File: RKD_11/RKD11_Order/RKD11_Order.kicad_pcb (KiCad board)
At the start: 2 copper layers, 99.4 x 99.4 mm, 140 parts, among them J1 Conn_01x06, J3 Qwiic_RA, SW1 RotaryEncoder_Switch, SW2 SW_Push, SW99 KEY_SWITCH, U1 ProMicro

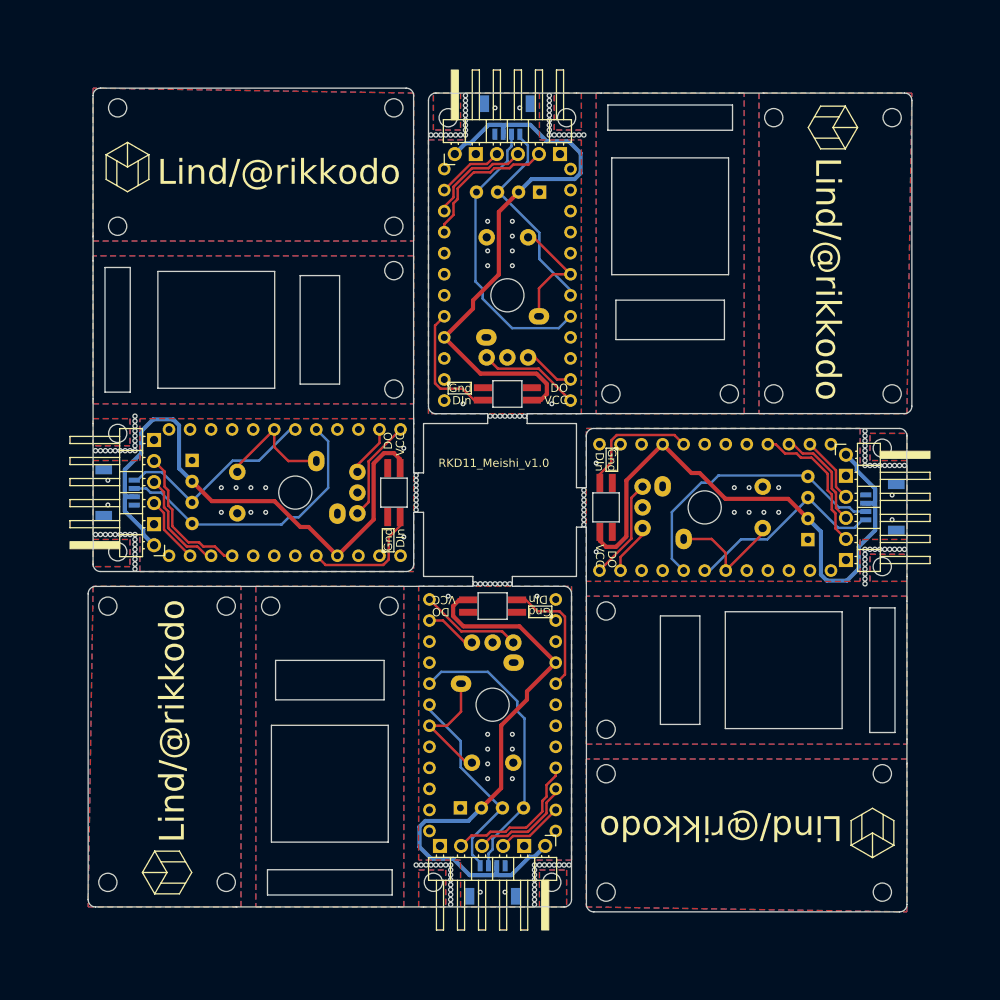
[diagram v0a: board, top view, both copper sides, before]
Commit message: Update
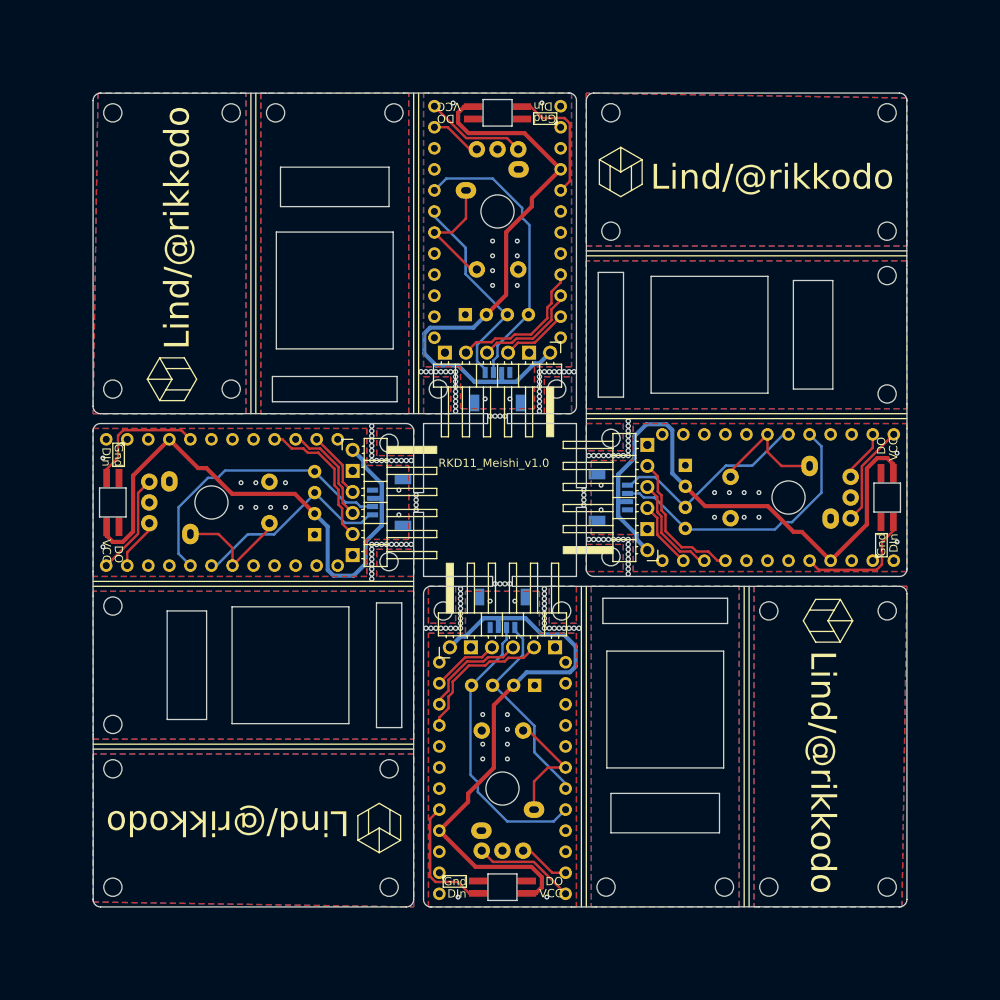
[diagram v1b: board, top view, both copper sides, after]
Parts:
- removed the J1 at (131.8, 58.0)
- removed the J1 at (95.5, 105.2)
- removed the J1 at (142.7, 141.5)
- removed the J1 at (179.0, 94.3)
- removed the J3 at (93.1, 98.8)
- removed the J3 at (181.4, 100.6)
- removed the J3 at (138.1, 55.6)
- removed the J3 at (136.3, 143.9)
- removed the LED1 at (124.4, 98.8)
- removed the LED1 at (138.1, 86.9)
- removed the LED1 at (136.3, 112.5)
- removed the LED1 at (150.0, 100.6)
- removed the LED3 at (157.8, 53.6)
- removed the LED3 at (91.1, 79.2)
- removed the LED3 at (116.7, 145.9)
- removed the LED3 at (183.4, 120.3)
- removed the OL1 at (192.9, 100.7)
- removed the OL1 at (138.2, 44.1)
- removed the OL1 at (136.2, 155.4)
- removed the OL1 at (81.6, 98.7)
- removed the REF** at (184.5, 105.7)
- removed the REF** at (143.2, 54.8)
- removed the REF** at (127.4, 143.8)
- removed the REF** at (93.2, 106.6)
- removed the REF** at (132.8, 55.7)
- removed the REF** at (127.1, 98.8)
- removed the REF** at (182.2, 105.7)
- removed the REF** at (92.3, 93.8)
- removed the REF** at (133.1, 53.6)
- removed the REF** at (181.3, 108.3)
- removed the REF** at (133.1, 52.4)
- removed the REF** at (185.7, 105.7)
- removed the REF** at (133.1, 51.2)
- removed the REF** at (93.2, 93.5)
- removed the REF** at (92.3, 59.5)
- removed the REF** at (145.3, 143.8)
- removed the REF** at (130.4, 55.7)
- removed the REF** at (182.2, 95.5)
- removed the REF** at (131.0, 143.8)
- removed the REF** at (144.7, 55.7)
- removed the REF** at (142.9, 143.8)
- removed the REF** at (131.3, 145.9)
- removed the REF** at (185.7, 95.5)
- removed the REF** at (89.9, 93.8)
- removed the REF** at (91.1, 93.8)
- removed the REF** at (93.2, 92.3)
- removed the REF** at (97.0, 144.7)
- removed the REF** at (181.3, 106.0)
- removed the REF** at (131.3, 144.7)
- removed the REF** at (136.3, 109.8)
- removed the REF** at (133.1, 54.8)
- removed the REF** at (181.3, 91.7)
- removed the REF** at (181.3, 107.2)
- removed the REF** at (143.2, 52.4)
- removed the REF** at (141.7, 143.8)
- removed the REF** at (131.3, 148.2)
- removed the REF** at (138.1, 89.6)
- removed the REF** at (141.4, 148.2)
- removed the REF** at (143.2, 51.2)
- removed the REF** at (89.9, 103.9)
- removed the REF** at (147.3, 100.6)
- removed the REF** at (131.3, 147.0)
- removed the REF** at (92.3, 103.9)
- removed the REF** at (141.4, 145.9)
- removed the REF** at (177.4, 54.8)
- removed the REF** at (183.4, 105.7)
- removed the REF** at (145.9, 55.7)
- removed the REF** at (181.3, 109.5)
- removed the REF** at (131.6, 55.7)
- removed the REF** at (181.3, 92.9)
- removed the REF** at (183.4, 95.5)
- removed the REF** at (144.1, 143.8)
- removed the REF** at (88.7, 103.9)
- removed the REF** at (181.3, 94.1)
- removed the REF** at (141.4, 147.0)
- removed the REF** at (141.4, 144.7)
- removed the REF** at (93.2, 91.1)
- removed the REF** at (93.2, 104.2)
- removed the REF** at (129.8, 143.8)
- removed the REF** at (181.3, 95.2)
- removed the REF** at (143.2, 53.6)
- removed the REF** at (129.2, 55.7)
- removed the REF** at (143.5, 55.7)
- removed the REF** at (182.2, 139.9)
- removed the REF** at (128.6, 143.8)
- removed the REF** at (91.1, 103.9)
- removed the REF** at (147.0, 55.7)
- removed the REF** at (88.7, 93.8)
- removed the REF** at (93.2, 89.9)
- removed the REF** at (184.5, 95.5)
- removed the REF** at (93.2, 107.8)
- removed the REF** at (93.2, 105.4)
- removed the Ref** at (184.5, 86.9)
- removed the Ref** at (170.3, 53.6)
- removed the Ref** at (150.6, 86.9)
- removed the Ref** at (124.4, 66.7)
- removed the Ref** at (91.1, 106.0)
- removed the Ref** at (184.5, 53.6)
- removed the Ref** at (150.0, 147.0)
- removed the Ref** at (183.4, 147.0)
- removed the Ref** at (170.3, 86.9)
- removed the Ref** at (91.1, 66.7)
- removed the Ref** at (89.9, 145.9)
- removed the Ref** at (150.0, 132.8)
- removed the Ref** at (124.4, 86.3)
- removed the Ref** at (143.5, 145.9)
- removed the Ref** at (123.8, 112.5)
- removed the Ref** at (124.4, 52.4)
- removed the Ref** at (131.0, 53.6)
- removed the Ref** at (150.0, 127.4)
- removed the Ref** at (145.3, 53.6)
- removed the Ref** at (164.9, 86.9)
- removed the Ref** at (91.1, 91.7)
- removed the Ref** at (109.5, 112.5)
- removed the Ref** at (104.2, 112.5)
- removed the Ref** at (150.0, 113.1)
- removed the Ref** at (183.4, 107.8)
- removed the Ref** at (129.2, 145.9)
- removed the Ref** at (124.4, 72.0)
- removed the Ref** at (89.9, 112.5)
- removed the Ref** at (104.2, 145.9)
- removed the Ref** at (183.4, 93.5)
- removed the Ref** at (91.1, 52.4)
- removed the Ref** at (183.4, 132.8)
- removed the SW1 at (138.1, 75.0)
- removed the SW1 at (112.5, 98.8)
- removed the SW1 at (161.9, 100.6)
- removed the SW1 at (136.3, 124.4)
- removed the SW2 at (161.9, 100.6)
- removed the SW2 at (112.5, 98.8)
- removed the SW2 at (136.3, 124.4)
- removed the SW2 at (138.1, 75.0)
- removed the SW99 at (103.0, 79.2)
- removed the SW99 at (116.7, 134.0)
- removed the SW99 at (171.5, 120.3)
- removed the SW99 at (157.8, 65.5)
- removed the U1 at (136.3, 124.4)
- removed the U1 at (112.5, 98.8)
- removed the U1 at (161.9, 100.6)
- removed the U1 at (138.1, 75.0)
- added J1: Conn_01x06, Connector_PinHeader_2.54mm:PinHeader_1x06_P2.54mm_Horizontal, F.Cu at (155.0, 105.8)
- added J1: Conn_01x06, Connector_PinHeader_2.54mm:PinHeader_1x06_P2.54mm_Horizontal, F.Cu at (119.4, 93.7)
- added J1: Conn_01x06, Connector_PinHeader_2.54mm:PinHeader_1x06_P2.54mm_Horizontal, F.Cu at (131.2, 117.5)
- added J1: Conn_01x06, Connector_PinHeader_2.54mm:PinHeader_1x06_P2.54mm_Horizontal, F.Cu at (143.3, 81.9)
- added J3: Qwiic_RA, SparkFun-Connector:JST_SMD_1.0mm-4_Black, B.Cu at (137.5, 115.1)
- added J3: Qwiic_RA, SparkFun-Connector:JST_SMD_1.0mm-4_Black, B.Cu at (121.8, 100.0)
- added J3: Qwiic_RA, SparkFun-Connector:JST_SMD_1.0mm-4_Black, B.Cu at (136.9, 84.3)
- added J3: Qwiic_RA, SparkFun-Connector:JST_SMD_1.0mm-4_Black, B.Cu at (152.6, 99.4)
- added LED1: LED_SK6812MINI-E, kbd_Parts:LED_SK6812MINI-E_UG, B.Cu at (136.9, 53.0)
- added LED1: LED_SK6812MINI-E, kbd_Parts:LED_SK6812MINI-E_UG, B.Cu at (90.5, 100.0)
- added LED1: LED_SK6812MINI-E, kbd_Parts:LED_SK6812MINI-E_UG, B.Cu at (137.5, 146.4)
- added LED1: LED_SK6812MINI-E, kbd_Parts:LED_SK6812MINI-E_UG, B.Cu at (184.0, 99.4)
- added LED3: LED_SK6812MINI-E, Rikkodo_FootPrint:rkd_KeyHall_3ox15, F.Cu at (123.8, 119.7)
- added LED3: LED_SK6812MINI-E, Rikkodo_FootPrint:rkd_KeyHall_3ox15, F.Cu at (117.3, 86.3)
- added LED3: LED_SK6812MINI-E, Rikkodo_FootPrint:rkd_KeyHall_3ox15, F.Cu at (150.6, 79.8)
- added LED3: LED_SK6812MINI-E, Rikkodo_FootPrint:rkd_KeyHall_3ox15, F.Cu at (157.2, 113.1)
- added OL1: OLED, BrownSugar_KBD:OLED_center_display, F.Cu at (137.6, 103.6)
- added OL1: OLED, BrownSugar_KBD:OLED_center_display, F.Cu at (136.8, 95.8)
- added OL1: OLED, BrownSugar_KBD:OLED_center_display, F.Cu at (133.3, 100.1)
- added OL1: OLED, BrownSugar_KBD:OLED_center_display, F.Cu at (141.1, 99.3)
- added REF**: rkd_cutdot_no_edgecut_1, Rikkodo_FootPrint:rkd_cutdot_no_edgecut_1, F.Cu at (149.4, 104.5)
- added REF**: rkd_LOGO, Rikkodo_FootPrint:rkd_LOGO, F.Cu at (151.8, 60.1)
- added REF**: rkd_cutdot_no_edgecut_1, Rikkodo_FootPrint:rkd_cutdot_no_edgecut_1, F.Cu at (131.9, 85.1)
- added REF**: rkd_cutdot_no_edgecut_1, Rikkodo_FootPrint:rkd_cutdot_no_edgecut_1, F.Cu at (131.6, 84.2)
- added REF**: rkd_cutdot_no_edgecut_1, Rikkodo_FootPrint:rkd_cutdot_no_edgecut_1, F.Cu at (148.2, 94.4)
- added REF**: rkd_cutdot_no_edgecut_1, Rikkodo_FootPrint:rkd_cutdot_no_edgecut_1, F.Cu at (142.6, 110.7)
- added REF**: rkd_cutdot_no_edgecut_1, Rikkodo_FootPrint:rkd_cutdot_no_edgecut_1, F.Cu at (152.7, 106.0)
- added REF**: rkd_cutdot_no_edgecut_1, Rikkodo_FootPrint:rkd_cutdot_no_edgecut_1, F.Cu at (126.2, 95.0)
- added REF**: rkd_cutdot_no_edgecut_1, Rikkodo_FootPrint:rkd_cutdot_no_edgecut_1, F.Cu at (123.8, 95.0)
- added REF**: rkd_cutdot_no_edgecut_1, Rikkodo_FootPrint:rkd_cutdot_no_edgecut_1, F.Cu at (152.7, 94.1)
- added REF**: rkd_cutdot_no_edgecut_1, Rikkodo_FootPrint:rkd_cutdot_no_edgecut_1, F.Cu at (151.8, 94.4)
- added REF**: rkd_cutdot_no_edgecut_1, Rikkodo_FootPrint:rkd_cutdot_no_edgecut_1, F.Cu at (151.8, 104.5)
- added REF**: rkd_LOGO, Rikkodo_FootPrint:rkd_LOGO, F.Cu at (97.6, 85.1)
- added REF**: rkd_cutdot_no_edgecut_1, Rikkodo_FootPrint:rkd_cutdot_no_edgecut_1, F.Cu at (131.9, 87.5)
- added REF**: rkd_cutdot_no_edgecut_1, Rikkodo_FootPrint:rkd_cutdot_no_edgecut_1, F.Cu at (131.9, 86.3)
- added REF**: rkd_cutdot_no_edgecut_1, Rikkodo_FootPrint:rkd_cutdot_no_edgecut_1, F.Cu at (122.6, 95.0)
- added REF**: rkd_cutdot_no_edgecut_1, Rikkodo_FootPrint:rkd_cutdot_no_edgecut_1, F.Cu at (150.6, 104.5)
- added REF**: rkd_cutdot_no_edgecut_1, Rikkodo_FootPrint:rkd_cutdot_no_edgecut_1, F.Cu at (129.8, 115.2)
- added REF**: rkd_cutdot_no_edgecut_1, Rikkodo_FootPrint:rkd_cutdot_no_edgecut_1, F.Cu at (145.3, 115.2)
- added REF**: rkd_cutdot_no_edgecut_1, Rikkodo_FootPrint:rkd_cutdot_no_edgecut_1, F.Cu at (121.7, 93.5)
- added REF**: rkd_cutdot_no_edgecut_1, Rikkodo_FootPrint:rkd_cutdot_no_edgecut_1, F.Cu at (131.0, 115.2)
- added REF**: rkd_cutdot_no_edgecut_1, Rikkodo_FootPrint:rkd_cutdot_no_edgecut_1, F.Cu at (122.6, 105.1)
- added REF**: rkd_cutdot_no_edgecut_1, Rikkodo_FootPrint:rkd_cutdot_no_edgecut_1, F.Cu at (128.6, 115.2)
- added REF**: rkd_cutdot_no_edgecut_1, Rikkodo_FootPrint:rkd_cutdot_no_edgecut_1, F.Cu at (144.7, 84.2)
- added REF**: rkd_cutdot_no_edgecut_1, Rikkodo_FootPrint:rkd_cutdot_no_edgecut_1, F.Cu at (145.9, 84.2)
- added REF**: rkd_cutdot_no_edgecut_1, Rikkodo_FootPrint:rkd_cutdot_no_edgecut_1, F.Cu at (142.0, 87.5)
- added REF**: rkd_cutdot, Rikkodo_FootPrint:rkd_cutdot, F.Cu at (136.9, 89.6)
- added REF**: rkd_cutdot_no_edgecut_1, Rikkodo_FootPrint:rkd_cutdot_no_edgecut_1, F.Cu at (152.7, 107.2)
- added REF**: rkd_cutdot_no_edgecut_1, Rikkodo_FootPrint:rkd_cutdot_no_edgecut_1, F.Cu at (152.7, 104.8)
- added REF**: rkd_cutdot_no_edgecut_1, Rikkodo_FootPrint:rkd_cutdot_no_edgecut_1, F.Cu at (150.6, 94.4)
- added REF**: rkd_cutdot_no_edgecut_1, Rikkodo_FootPrint:rkd_cutdot_no_edgecut_1, F.Cu at (121.7, 106.6)
- added REF**: rkd_cutdot_no_edgecut_1, Rikkodo_FootPrint:rkd_cutdot_no_edgecut_1, F.Cu at (142.9, 115.2)
- added REF**: rkd_cutdot_no_edgecut_1, Rikkodo_FootPrint:rkd_cutdot_no_edgecut_1, F.Cu at (142.6, 111.9)
- added REF**: rkd_cutdot_no_edgecut_1, Rikkodo_FootPrint:rkd_cutdot_no_edgecut_1, F.Cu at (130.4, 84.2)
- added REF**: rkd_cutdot_no_edgecut_1, Rikkodo_FootPrint:rkd_cutdot_no_edgecut_1, F.Cu at (132.5, 111.9)
- added REF**: rkd_cutdot_no_edgecut_1, Rikkodo_FootPrint:rkd_cutdot_no_edgecut_1, F.Cu at (132.5, 113.1)
- added REF**: rkd_cutdot_no_edgecut_1, Rikkodo_FootPrint:rkd_cutdot_no_edgecut_1, F.Cu at (123.8, 105.1)
- added REF**: rkd_cutdot_no_edgecut_1, Rikkodo_FootPrint:rkd_cutdot_no_edgecut_1, F.Cu at (132.5, 110.7)
- added REF**: rkd_cutdot_no_edgecut_1, Rikkodo_FootPrint:rkd_cutdot_no_edgecut_1, F.Cu at (125.0, 95.0)
- added REF**: rkd_cutdot_no_edgecut_1, Rikkodo_FootPrint:rkd_cutdot_no_edgecut_1, F.Cu at (121.7, 94.7)
- added REF**: rkd_cutdot_no_edgecut_1, Rikkodo_FootPrint:rkd_cutdot_no_edgecut_1, F.Cu at (144.1, 115.2)
- added REF**: rkd_cutdot_no_edgecut_1, Rikkodo_FootPrint:rkd_cutdot_no_edgecut_1, F.Cu at (126.2, 105.1)
- added REF**: rkd_cutdot_no_edgecut_1, Rikkodo_FootPrint:rkd_cutdot_no_edgecut_1, F.Cu at (121.7, 91.1)
- added REF**: rkd_cutdot_no_edgecut_1, Rikkodo_FootPrint:rkd_cutdot_no_edgecut_1, F.Cu at (121.7, 105.4)
- added REF**: rkd_cutdot_no_edgecut_1, Rikkodo_FootPrint:rkd_cutdot_no_edgecut_1, F.Cu at (142.6, 113.1)
- added REF**: rkd_cutdot, Rikkodo_FootPrint:rkd_cutdot, F.Cu at (127.1, 100.0)
- added REF**: rkd_cutdot_no_edgecut_1, Rikkodo_FootPrint:rkd_cutdot_no_edgecut_1, F.Cu at (132.2, 115.2)
- added REF**: rkd_LOGO, Rikkodo_FootPrint:rkd_LOGO, F.Cu at (176.8, 114.3)
- added REF**: rkd_cutdot_no_edgecut_1, Rikkodo_FootPrint:rkd_cutdot_no_edgecut_1, F.Cu at (142.0, 85.1)
- added REF**: rkd_cutdot_no_edgecut_1, Rikkodo_FootPrint:rkd_cutdot_no_edgecut_1, F.Cu at (125.0, 105.1)
- added REF**: rkd_cutdot_no_edgecut_1, Rikkodo_FootPrint:rkd_cutdot_no_edgecut_1, F.Cu at (143.5, 84.2)
- added REF**: rkd_cutdot_no_edgecut_1, Rikkodo_FootPrint:rkd_cutdot_no_edgecut_1, F.Cu at (152.7, 90.5)
- added REF**: rkd_LOGO, Rikkodo_FootPrint:rkd_LOGO, F.Cu at (122.6, 139.3)
- added REF**: rkd_cutdot_no_edgecut_1, Rikkodo_FootPrint:rkd_cutdot_no_edgecut_1, F.Cu at (142.0, 88.7)
- added REF**: rkd_cutdot_no_edgecut_1, Rikkodo_FootPrint:rkd_cutdot_no_edgecut_1, F.Cu at (142.0, 86.3)
- added REF**: rkd_cutdot_no_edgecut_1, Rikkodo_FootPrint:rkd_cutdot_no_edgecut_1, F.Cu at (131.9, 88.7)
- added REF**: rkd_cutdot_no_edgecut_1, Rikkodo_FootPrint:rkd_cutdot_no_edgecut_1, F.Cu at (146.4, 115.2)
- added REF**: rkd_cutdot_no_edgecut_1, Rikkodo_FootPrint:rkd_cutdot_no_edgecut_1, F.Cu at (121.7, 107.8)
- added REF**: rkd_cutdot_no_edgecut_1, Rikkodo_FootPrint:rkd_cutdot_no_edgecut_1, F.Cu at (121.7, 92.3)
- added REF**: rkd_cutdot_no_edgecut_1, Rikkodo_FootPrint:rkd_cutdot_no_edgecut_1, F.Cu at (142.6, 114.3)
- added REF**: rkd_cutdot_no_edgecut_1, Rikkodo_FootPrint:rkd_cutdot_no_edgecut_1, F.Cu at (148.2, 104.5)
- added REF**: rkd_cutdot_no_edgecut_1, Rikkodo_FootPrint:rkd_cutdot_no_edgecut_1, F.Cu at (149.4, 94.4)
- added REF**: rkd_cutdot_no_edgecut_1, Rikkodo_FootPrint:rkd_cutdot_no_edgecut_1, F.Cu at (121.7, 108.9)
- added REF**: rkd_cutdot, Rikkodo_FootPrint:rkd_cutdot, F.Cu at (147.3, 99.4)
- added REF**: rkd_cutdot_no_edgecut_1, Rikkodo_FootPrint:rkd_cutdot_no_edgecut_1, F.Cu at (152.7, 108.3)
- added REF**: rkd_cutdot_no_edgecut_1, Rikkodo_FootPrint:rkd_cutdot_no_edgecut_1, F.Cu at (152.7, 92.9)
- added REF**: rkd_cutdot_no_edgecut_1, Rikkodo_FootPrint:rkd_cutdot_no_edgecut_1, F.Cu at (128.0, 84.2)
- added REF**: rkd_cutdot_no_edgecut_1, Rikkodo_FootPrint:rkd_cutdot_no_edgecut_1, F.Cu at (152.7, 91.7)
- added REF**: rkd_cutdot_no_edgecut_1, Rikkodo_FootPrint:rkd_cutdot_no_edgecut_1, F.Cu at (132.5, 114.3)
- added REF**: rkd_cutdot, Rikkodo_FootPrint:rkd_cutdot, F.Cu at (137.5, 109.8)
- added REF**: rkd_cutdot_no_edgecut_1, Rikkodo_FootPrint:rkd_cutdot_no_edgecut_1, F.Cu at (129.2, 84.2)
- added REF**: rkd_cutdot_no_edgecut_1, Rikkodo_FootPrint:rkd_cutdot_no_edgecut_1, F.Cu at (142.3, 84.2)
- added Ref**: Val**, kbd_Hole:m2_Screw_Hole, F.Cu at (90.5, 53.0)
- added Ref**: Val**, kbd_Hole:m2_Screw_Hole, F.Cu at (90.5, 132.2)
- added Ref**: Val**, kbd_Hole:m2_Screw_Hole, F.Cu at (150.6, 53.0)
- added Ref**: Val**, kbd_Hole:m2_Screw_Hole, F.Cu at (123.8, 146.4)
- added Ref**: Val**, kbd_Hole:m2_Screw_Hole, F.Cu at (124.4, 53.0)
- added Ref**: Val**, kbd_Hole:m2_Screw_Hole, F.Cu at (164.3, 146.4)
- added Ref**: Val**, kbd_Hole:m2_Screw_Hole, F.Cu at (183.9, 72.6)
- added Ref**: Val**, kbd_Hole:m2_Screw_Hole, F.Cu at (169.7, 113.1)
- added Ref**: Val**, kbd_Hole:m2_Screw_Hole, F.Cu at (144.1, 86.3)
- added Ref**: Val**, kbd_Hole:m2_Screw_Hole, F.Cu at (123.8, 92.9)
- added Ref**: Val**, kbd_Hole:m2_Screw_Hole, F.Cu at (150.6, 92.3)
- added Ref**: Val**, kbd_Hole:m2_Screw_Hole, F.Cu at (90.5, 112.5)
- added Ref**: Val**, kbd_Hole:m2_Screw_Hole, F.Cu at (183.9, 67.3)
- added Ref**: Val**, kbd_Hole:m2_Screw_Hole, F.Cu at (184.0, 113.1)
- added Ref**: Val**, kbd_Hole:m2_Screw_Hole, F.Cu at (123.8, 107.2)
- added Ref**: Val**, kbd_Hole:m2_Screw_Hole, F.Cu at (184.0, 146.4)
- added Ref**: Val**, kbd_Hole:m2_Screw_Hole, F.Cu at (144.7, 113.1)
- added Ref**: Val**, kbd_Hole:m2_Screw_Hole, F.Cu at (150.0, 146.4)
- added Ref**: Val**, kbd_Hole:m2_Screw_Hole, F.Cu at (123.8, 132.2)
- added Ref**: Val**, kbd_Hole:m2_Screw_Hole, F.Cu at (150.6, 106.6)
- added Ref**: Val**, kbd_Hole:m2_Screw_Hole, F.Cu at (90.5, 86.3)
- added Ref**: Val**, kbd_Hole:m2_Screw_Hole, F.Cu at (169.7, 146.4)
- added Ref**: Val**, kbd_Hole:m2_Screw_Hole, F.Cu at (104.8, 53.0)
- added Ref**: Val**, kbd_Hole:m2_Screw_Hole, F.Cu at (183.9, 86.9)
- added Ref**: Val**, kbd_Hole:m2_Screw_Hole, F.Cu at (104.8, 86.3)
- added Ref**: Val**, kbd_Hole:m2_Screw_Hole, F.Cu at (129.8, 86.3)
- added Ref**: Val**, kbd_Hole:m2_Screw_Hole, F.Cu at (130.4, 113.1)
- added Ref**: Val**, kbd_Hole:m2_Screw_Hole, F.Cu at (110.1, 53.0)
- added Ref**: Val**, kbd_Hole:m2_Screw_Hole, F.Cu at (183.9, 53.0)
- added Ref**: Val**, kbd_Hole:m2_Screw_Hole, F.Cu at (150.6, 67.3)
- added Ref**: Val**, kbd_Hole:m2_Screw_Hole, F.Cu at (90.5, 126.8)
- added Ref**: Val**, kbd_Hole:m2_Screw_Hole, F.Cu at (90.5, 146.4)
- added SW1: RotaryEncoder_Switch, BrownSugar_KBD:RotaryEncoder_EC11-Switch, F.Cu at (102.4, 100.0)
- added SW1: RotaryEncoder_Switch, BrownSugar_KBD:RotaryEncoder_EC11-Switch, F.Cu at (172.0, 99.4)
- added SW1: RotaryEncoder_Switch, BrownSugar_KBD:RotaryEncoder_EC11-Switch, F.Cu at (136.9, 64.9)
- added SW1: RotaryEncoder_Switch, BrownSugar_KBD:RotaryEncoder_EC11-Switch, F.Cu at (137.5, 134.5)
- added SW2: SW_Push, kbd_SW:CherryMX_Solder_1u, F.Cu at (137.5, 134.5)
- added SW2: SW_Push, kbd_SW:CherryMX_Solder_1u, F.Cu at (136.9, 64.9)
- added SW2: SW_Push, kbd_SW:CherryMX_Solder_1u, F.Cu at (102.4, 100.0)
- added SW2: SW_Push, kbd_SW:CherryMX_Solder_1u, F.Cu at (172.0, 99.4)
- added SW99: KEY_SWITCH, kbd_SW_Hole:SW_Hole_1u, F.Cu at (111.9, 119.7)
- added SW99: KEY_SWITCH, kbd_SW_Hole:SW_Hole_1u, F.Cu at (162.5, 79.8)
- added SW99: KEY_SWITCH, kbd_SW_Hole:SW_Hole_1u, F.Cu at (157.2, 125.0)
- added SW99: KEY_SWITCH, kbd_SW_Hole:SW_Hole_1u, F.Cu at (117.3, 74.4)
- added U1: ProMicro, BrownSugar_KBD:ProMicro_r, B.Cu at (136.9, 64.9)
- added U1: ProMicro, BrownSugar_KBD:ProMicro_r, B.Cu at (137.5, 134.5)
- added U1: ProMicro, BrownSugar_KBD:ProMicro_r, B.Cu at (172.0, 99.4)
- added U1: ProMicro, BrownSugar_KBD:ProMicro_r, B.Cu at (102.4, 100.0)
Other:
- board size 99.4 x 99.4 mm -> 98.2 x 98.2 mm
